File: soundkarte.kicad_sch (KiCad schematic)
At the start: 311 parts, among them J1 JTAG, J2 DB9, J3 Conn_01x05_Pin, J4 Conn_01x06_Pin, J5 Conn_01x08_Pin, J6 LSP R, J7 Sub, J8 LSP L, Q1 Q_NPN_BEC, Q2 BC807, Q3 BC807, U1 DSP56364, U12 LM78M05_TO252, U13 Opamp_Dual, U14 74HC74, U15 TS274CD, U2 28F640, U3 74LS393, U4 74HC14, U8 LD1086D2M33TR, U9 LD1086D2M33TR, X1 SG-8002JC

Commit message: loeschen
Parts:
- removed C1, C2, C3, C4, C47, C48, C49, C5, C50, C51, C6, C7, C8: 220 35G, Capacitor_SMD:CP_Elec_10x10.5, symbol Device:C_Polarized
- removed C10, C11, C12, C13, C14, C15, C16, C17, C18, C27, C28, C29, C30, C31, C32, C33, C34, C35, C36, C37, C38, C39, C40, C41, C42, C43, C44, C45, C46, C55, C56, C57, C61, C62, C63, C64, C65, C66, C67, C68, C69, C70, C73, C74, C9: C, Capacitor_SMD:C_0805_2012Metric, symbol Device:C
- removed C19, C20, C21, C22, C23, C24, C25, C26, C52, C53, C54: 22 35G, Capacitor_SMD:CP_Elec_6.3x3, symbol Device:C_Polarized
- removed C58, C59, C60, C71, C72, C75, C76, C77, C78, C79: C, Capacitor_SMD:C_1206_3216Metric, symbol Device:C
- removed D1, D2, D3, D4: LED, LED_SMD:LED_PLCC-2_3.4x3.0mm_AK, symbol Device:LED
- removed D5: D, Diode_SMD:D_1812_4532Metric, symbol Device:D
- removed FID2, FID3: Fiducial, Fiducial:Fiducial_0.75mm_Mask2.25mm, symbol Mechanical:Fiducial
- removed H5, H6: MountingHole, MountingHole:MountingHole_4mm, symbol Mechanical:MountingHole
- removed H7: MountingHole_Pad, MountingHole:MountingHole_4mm_Pad, symbol Mechanical:MountingHole_Pad
- removed J1: JTAG, Soundkarte:PinHeader_2x7_P1.27mm_Vertical_SMD_Pin1Left, symbol Connector_Generic:Conn_02x07_Odd_Even
- removed J2: DB9, Connector_Dsub:DSUB-9_Female_Vertical_P2.77x2.84mm, symbol Connector:Conn_01x09_Socket
- removed J3: Conn_01x05_Pin, Connector_PinHeader_2.54mm:PinHeader_1x05_P2.54mm_Vertical, symbol Connector:Conn_01x05_Pin
- removed J4: Conn_01x06_Pin, Connector_PinHeader_2.54mm:PinHeader_1x06_P2.54mm_Vertical, symbol Connector:Conn_01x06_Pin
- removed J5: Conn_01x08_Pin, Connector_PinHeader_2.54mm:PinHeader_1x08_P2.54mm_Vertical, symbol Connector:Conn_01x08_Pin
- removed J6: LSP R, Connector_PinHeader_2.54mm:PinHeader_1x02_P2.54mm_Vertical, symbol Connector:Conn_01x02_Pin
- removed J7: Sub, Connector_PinHeader_2.54mm:PinHeader_1x02_P2.54mm_Vertical, symbol Connector:Conn_01x02_Pin
- removed J8: LSP L, Connector_PinHeader_2.54mm:PinHeader_1x02_P2.54mm_Vertical, symbol Connector:Conn_01x02_Pin
- removed JP4: Mcdac, Jumper:SolderJumper-2_P1.3mm_Open_Pad1.0x1.5mm, symbol Jumper:Jumper_2_Open
- removed L1: L_Coupled, Inductor_THT:Choke_Schaffner_RN212-04-12.5x18.0mm, symbol Device:L_Coupled
- removed Q1: Q_NPN_BEC, Package_TO_SOT_SMD:SOT-23-3, symbol Device:Q_NPN_BEC
- removed Q2, Q3: BC807, Package_TO_SOT_SMD:SOT-23-3, symbol Device:Q_PNP_BEC
- removed R1, R10, R11, R12, R13, R14, R15, R16, R17, R18, R19, R2, R20, R21, R22, R23, R24, R25, R26, R27, R28, R29, R3, R30, R31, R34, R35, R36, R37, R38, R4, R44, R45, R46, R49, R5, R51, R52, R53, R54, R55, R56, R57, R58, R6, R7, R8, R9: R, Resistor_SMD:R_0805_2012Metric, symbol Device:R
- removed R32: 0, Resistor_SMD:R_0805_2012Metric, symbol Device:R
- removed R33, R39, R40, R41, R42, R43, R50: 10k, Resistor_SMD:R_0805_2012Metric, symbol Device:R
- removed R47: log, Potentiometer_THT:Potentiometer_ACP_CA6-H2,5_Horizontal, symbol Device:R_Potentiometer
- removed R48: lin, Potentiometer_THT:Potentiometer_ACP_CA6-H2,5_Horizontal, symbol Device:R_Potentiometer
- removed R59, R60, R61, R62, R63, R64: R, Resistor_SMD:R_0603_1608Metric, symbol Device:R
- removed TP10, TP100, TP101, TP102, TP103, TP104, TP105, TP106, TP107, TP108, TP110, TP111, TP112, TP113, TP114, TP115, TP116, TP117, TP118, TP119, TP120, TP121, TP122, TP21, TP50, TP51, TP53, TP54, TP55, TP56, TP57, TP59, TP60, TP61, TP62, TP64, TP65, TP67, TP68, TP70, TP72, TP74, TP75, TP76, TP77, TP78, TP79, TP8, TP80, TP81, TP82, TP83, TP84, TP85, TP86, TP9, TP91, TP93, TP94, TP95, TP96, TP97, TP98, TP99: TestPoint, TestPoint:TestPoint_Pad_D1.0mm, symbol Connector:TestPoint
- removed U1: DSP56364, Package_QFP:LQFP-100_14x14mm_P0.5mm, symbol Soundkarte:DSP56364
- removed U10, U11: ~, Package_SO:SSOP-28_5.3x10.2mm_P0.65mm, symbol Soundkarte:PCM1716
- removed U12: LM78M05_TO252, Package_TO_SOT_SMD:TO-252-2, symbol Regulator_Linear:LM78M05_TO252
- removed U13: Opamp_Dual, Package_SO:SO-8_3.9x4.9mm_P1.27mm, symbol Device:Opamp_Dual
- removed U14: 74HC74, Package_SO:TSSOP-14_4.4x5mm_P0.65mm, symbol 74xx:74HC74
- removed U15: TS274CD, Package_SO:SO-14_3.9x8.65mm_P1.27mm, symbol Amplifier_Operational:TLC274
- removed U2: 28F640, Package_SO:TSOP-I-56_18.4x14mm_P0.5mm, symbol Soundkarte:JS28F640
- removed U3: 74LS393, Package_SO:SO-14_3.9x8.65mm_P1.27mm, symbol 74xx:74LS393
- removed U4: 74HC14, Package_SO:TSSOP-14_4.4x5mm_P0.65mm, symbol 74xx:74HC14
- removed U5, U6, U7: ~, Package_SO:Infineon_PG-DSO-20-87, symbol Soundkarte:TDA7391PD
- removed U8, U9: LD1086D2M33TR, Package_TO_SOT_SMD:TO-263-3_TabPin2, symbol Regulator_Linear:LD1086D2M33TR
- removed X1: SG-8002JC, Oscillator:Oscillator_SMD_SeikoEpson_SG8002JC-4Pin_10.5x5.0mm, symbol Oscillator:SG-8002JC
- added J1: Data, Connector_FFC-FPC:TE_84952-8_1x08-1MP_P1.0mm_Horizontal, symbol Connector_Generic_MountingPin:Conn_01x08_MountingPin
- added J10: Address, Connector_FFC-FPC:TE_2-84952-8_1x28-1MP_P1.0mm_Horizontal, symbol Connector_Generic_MountingPin:Conn_01x28_MountingPin
- added J2: Control, Connector_FFC-FPC:TE_84952-8_1x08-1MP_P1.0mm_Horizontal, symbol Connector_Generic_MountingPin:Conn_01x08_MountingPin
- added J4: Power, Connector_FFC-FPC:TE_84952-8_1x08-1MP_P1.0mm_Horizontal, symbol Connector_Generic_MountingPin:Conn_01x08_MountingPin
- added J5: 1-28, Connector_FFC-FPC:TE_2-84952-8_1x28-1MP_P1.0mm_Horizontal, symbol Connector_Generic_MountingPin:Conn_01x28_MountingPin
- added J6: JTAG, Connector_FFC-FPC:TE_84952-8_1x08-1MP_P1.0mm_Horizontal, symbol Connector_Generic_MountingPin:Conn_01x08_MountingPin
- added J7: 29-56, Connector_FFC-FPC:TE_2-84952-8_1x28-1MP_P1.0mm_Horizontal, symbol Connector_Generic_MountingPin:Conn_01x28_MountingPin
- added J8: Main Power, Connector_Wire:SolderWire-0.25sqmm_1x02_P4.5mm_D0.65mm_OD2mm_Relief, symbol Connector_Generic:Conn_01x02
- added J9: Aux Power, Connector_Wire:SolderWire-0.25sqmm_1x02_P4.5mm_D0.65mm_OD2mm_Relief, symbol Connector_Generic:Conn_01x02
- TP1, TP109, TP11, TP12, TP13, TP14, TP15, TP16, TP17, TP18, TP19, TP2, TP20, TP22, TP23, TP24, TP25, TP26, TP27, TP28, TP29, TP3, TP30, TP31, TP32, TP33, TP34, TP35, TP36, TP37, TP38, TP39, TP4, TP40, TP41, TP42, TP43, TP44, TP45, TP47, TP48, TP49, TP5, TP52, TP58, TP6, TP63, TP66, TP69, TP7, TP71, TP73, TP87, TP88, TP89, TP90, TP92: footprint TestPoint:TestPoint_Pad_D1.0mm -> TestPoint:TestPoint_THTPad_D2.0mm_Drill1.0mm
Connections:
- net +12V: now also J8.1 (Pin_1)
- net +3.3V: now also TP58.1, J4.4 (Pin_4), J4.5 (Pin_5), J4.7 (Pin_7), J5.9 (Pin_9), J6.1 (Pin_1)
- net +5V: now also J9.1 (Pin_1)
- net A0: now also J10.3 (Pin_3), J7.4 (Pin_4)
- net A1: now also J10.4 (Pin_4), J5.28 (Pin_28)
- net A10: now also J10.13 (Pin_13), J5.18 (Pin_18)
- net A11: now also J10.14 (Pin_14), J5.17 (Pin_17)
- net A12: now also J10.15 (Pin_15), J5.13 (Pin_13)
- net A13: now also J10.16 (Pin_16), J5.12 (Pin_12)
- net A14: now also J10.17 (Pin_17), J5.11 (Pin_11)
- net A15: now also J10.18 (Pin_18), J5.10 (Pin_10)
- net A16: now also J10.19 (Pin_19), J5.8 (Pin_8)
- net A17: now also J10.20 (Pin_20), J5.7 (Pin_7)
- net A18: now also J10.21 (Pin_21), J5.6 (Pin_6)
- net A19: now also J10.22 (Pin_22), J5.5 (Pin_5)
- net A2: now also J10.5 (Pin_5), J5.27 (Pin_27)
- net A24: now also J10.27 (Pin_27), J7.28 (Pin_28)
- net A3: now also J10.6 (Pin_6), J5.26 (Pin_26)
- net A4: now also J10.7 (Pin_7), J5.25 (Pin_25)
- net A5: now also J10.8 (Pin_8), J5.24 (Pin_24)
- net A6: now also J10.9 (Pin_9), J5.23 (Pin_23)
- net A7: now also J10.10 (Pin_10), J5.22 (Pin_22)
- net A8: now also J10.11 (Pin_11), J5.20 (Pin_20)
- net A9: now also J10.12 (Pin_12), J5.19 (Pin_19)
- net D0: now also J1.1 (Pin_1), J7.5 (Pin_5)
- net D1: now also J1.2 (Pin_2), J7.7 (Pin_7)
- net D2: now also J1.3 (Pin_3), J7.10 (Pin_10)
- net D3: now also J1.4 (Pin_4), J7.12 (Pin_12)
- net D4: now also J1.5 (Pin_5), J7.16 (Pin_16)
- net D5: now also J1.6 (Pin_6), J7.18 (Pin_18)
- net D6: now also J1.7 (Pin_7), J7.21 (Pin_21)
- net D7: now also J1.8 (Pin_8), J7.23 (Pin_23)
- net GND: now also J1.MP (MountPin), J10.1 (Pin_1), J10.2 (Pin_2), J10.28 (Pin_28), J10.MP (MountPin), J2.3 (Pin_3), J2.MP (MountPin), J4.1 (Pin_1), J4.2 (Pin_2), J4.3 (Pin_3), J4.MP (MountPin), J5.2 (Pin_2), J5.21 (Pin_21), J5.MP (MountPin), J6.3 (Pin_3), J6.7 (Pin_7), J6.MP (MountPin), J7.14 (Pin_14), J7.20 (Pin_20), J7.MP (MountPin), J8.2 (Pin_2), J9.2 (Pin_2)
- net GPIO0: now also J10.23 (Pin_23), J5.4 (Pin_4)
- net GPIO1: now also J10.24 (Pin_24), J5.3 (Pin_3)
- net GPIO2: now also J10.25 (Pin_25), J5.1 (Pin_1)
- net GPIO3: now also J10.26 (Pin_26), J7.2 (Pin_2)
- net RESET: now also J2.7 (Pin_7), J5.16 (Pin_16)
- net TCK: now also J6.4 (Pin_4)
- net TDI: now also J6.2 (Pin_2)
- net TDO: now also J6.6 (Pin_6)
- net TMS: now also J6.8 (Pin_8)
- net MODD: now reaches JP3.1 (A), TP18.1
- net at TP22.1: now also J2.6 (Pin_6), J7.26 (Pin_26)
- net at TP23.1: now also J2.5 (Pin_5), J7.27 (Pin_27)
- net at TP49.1: now also J4.6 (Pin_6), J5.15 (Pin_15)
- net at TP66.1: now also J2.8 (Pin_8), J7.25 (Pin_25)
- net MODA: now reaches JP1.1 (A), TP20.1
- net MODB: now reaches JP2.1 (A), TP19.1
- net at TP47.1: now also J2.2 (Pin_2), J5.14 (Pin_14)
- new net: J2.1 (Pin_1), J2.4 (Pin_4), J7.1 (Pin_1), J7.3 (Pin_3)
- new net: J4.8 (Pin_8), J7.15 (Pin_15), J7.9 (Pin_9)
- no-connect marks 18 -> 0
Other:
- moved on the sheet: TP1, TP11, TP12, TP13, TP14, TP15, TP2, TP3, TP4, TP42, TP43, TP44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

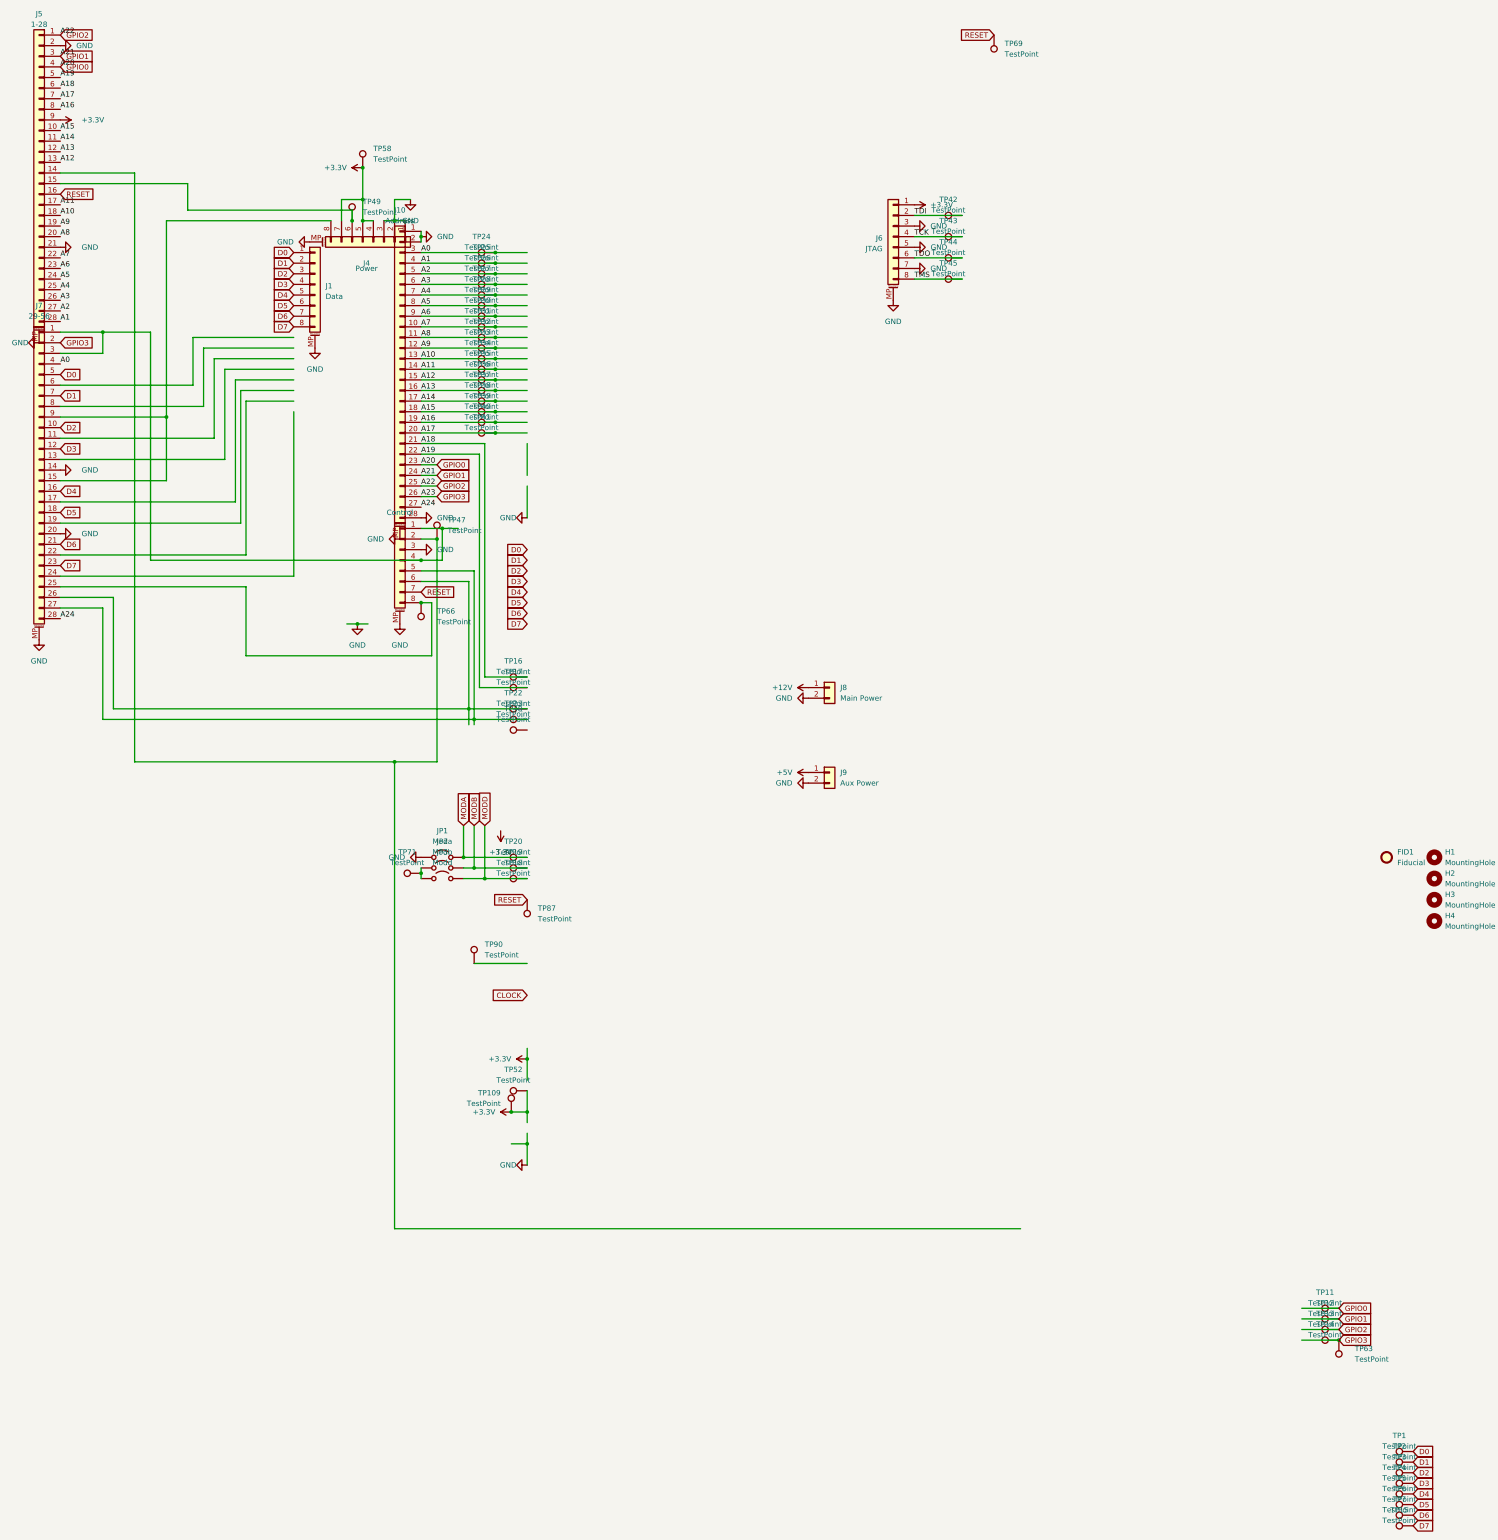
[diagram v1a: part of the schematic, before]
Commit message: teensy
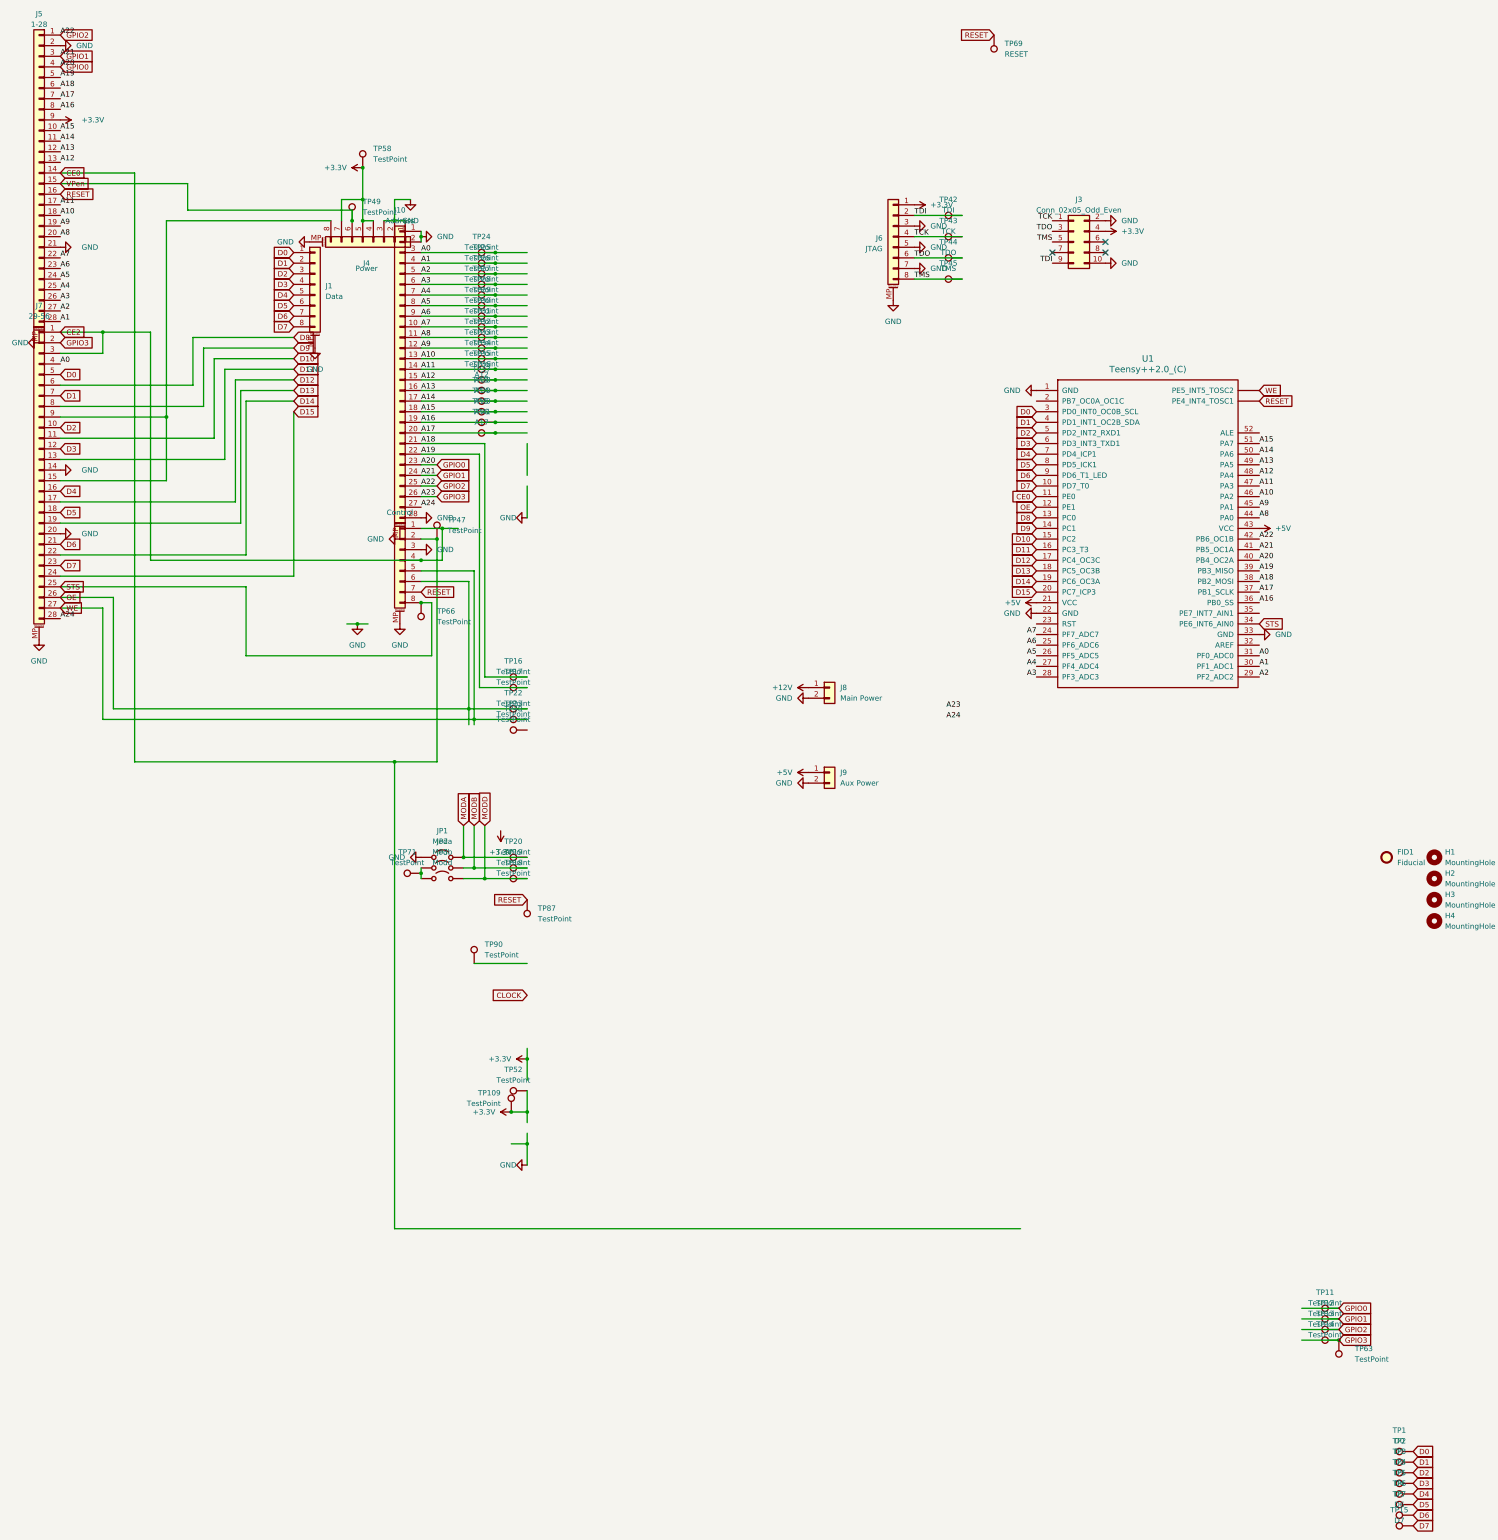
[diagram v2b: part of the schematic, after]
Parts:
- added J3: Conn_02x05_Odd_Even, Connector_PinHeader_2.54mm:PinHeader_2x05_P2.54mm_Vertical, symbol Connector_Generic:Conn_02x05_Odd_Even
- added U1: Teensy++2.0_(C), Soundkarte:Teensy2.0++, symbol teensy:Teensy++2.0_(C)
- TP1: value TestPoint -> D0
- TP15: value TestPoint -> D7
- TP2: value TestPoint -> D1
- TP3: value TestPoint -> D2
- TP36: value TestPoint -> A12
- TP37: value TestPoint -> A13
- TP38: value TestPoint -> A14
- TP39: value TestPoint -> A15
- TP4: value TestPoint -> D3
- TP40: value TestPoint -> A16
- TP41: value TestPoint -> A17
- TP42: value TestPoint -> TDI
- TP43: value TestPoint -> TCK
- TP44: value TestPoint -> TDO
- TP45: value TestPoint -> TMS
- TP5: value TestPoint -> D4
- TP6: value TestPoint -> D5
- TP69: value TestPoint -> RESET
- TP7: value TestPoint -> D6
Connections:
- net +3.3V: now also J3.4 (Pin_4)
- net +5V: now also U1.21 (VCC), U1.43 (VCC)
- net A0: now also U1.31 (PF0_ADC0)
- net A1: now also U1.30 (PF1_ADC1)
- net A10: now also U1.46 (PA2)
- net A11: now also U1.47 (PA3)
- net A12: now also U1.48 (PA4)
- net A13: now also U1.49 (PA5)
- net A14: now also U1.50 (PA6)
- net A15: now also U1.51 (PA7)
- net A16: now also U1.36 (PB0_SS)
- net A17: now also U1.37 (PB1_SCLK)
- net A18: now also U1.38 (PB2_MOSI)
- net A19: now also U1.39 (PB3_MISO)
- net A2: now also U1.29 (PF2_ADC2)
- net A3: now also U1.28 (PF3_ADC3)
- net A4: now also U1.27 (PF4_ADC4)
- net A5: now also U1.26 (PF5_ADC5)
- net A6: now also U1.25 (PF6_ADC6)
- net A7: now also U1.24 (PF7_ADC7)
- net A8: now also U1.44 (PA0)
- net A9: now also U1.45 (PA1)
- net D0: now also U1.3 (PD0_INT0_OC0B_SCL)
- net D1: now also U1.4 (PD1_INT1_OC2B_SDA)
- net D2: now also U1.5 (PD2_INT2_RXD1)
- net D3: now also U1.6 (PD3_INT3_TXD1)
- net D4: now also U1.7 (PD4_ICP1)
- net D5: now also U1.8 (PD5_ICK1)
- net D6: now also U1.9 (PD6_T1_LED)
- net D7: now also U1.10 (PD7_T0)
- net GND: now also J6.5 (Pin_5), J3.10 (Pin_10), J3.2 (Pin_2), U1.1 (GND), U1.22 (GND), U1.33 (GND)
- net GPIO0: now also U1.40 (PB4_OC2A)
- net GPIO1: now also U1.41 (PB5_OC1A)
- net GPIO2: now also U1.42 (PB6_OC1B)
- net RESET: now also U1.~ (PE4_INT4_TOSC1)
- net TCK: now also J3.1 (Pin_1)
- net TDI: now also J3.9 (Pin_9)
- net TDO: now also J3.3 (Pin_3)
- net TMS: now also J3.5 (Pin_5)
- net CE0: now reaches J2.2 (Pin_2), J5.14 (Pin_14), TP47.1
- net CE0: now also U1.11 (PE0)
- net VPen: now reaches J4.6 (Pin_6), J5.15 (Pin_15), TP49.1
- net CE2: now reaches J2.1 (Pin_1), J2.4 (Pin_4), J7.1 (Pin_1), J7.3 (Pin_3)
- net WE: now reaches J2.5 (Pin_5), J7.27 (Pin_27), TP23.1
- net WE: now also U1.~ (PE4_INT4_TOSC1)
- net OE: now reaches J2.6 (Pin_6), J7.26 (Pin_26), TP22.1
- net OE: now also U1.12 (PE1)
- net STS: now reaches J2.8 (Pin_8), J7.25 (Pin_25), TP66.1
- net STS: now also U1.34 (PE6_INT6_AIN0)
- net D10: now reaches J7.11 (Pin_11)
- net D10: now also U1.15 (PC2)
- net D11: now reaches J7.13 (Pin_13)
- net D11: now also U1.16 (PC3_T3)
- net D12: now reaches J7.17 (Pin_17)
- net D12: now also U1.17 (PC4_OC3C)
- net D13: now reaches J7.19 (Pin_19)
- net D13: now also U1.18 (PC5_OC3B)
- net D14: now reaches J7.22 (Pin_22)
- net D14: now also U1.19 (PC6_OC3A)
- net D15: now reaches J7.24 (Pin_24)
- net D15: now also U1.20 (PC7_ICP3)
- net D8: now reaches J7.6 (Pin_6)
- net D8: now also U1.13 (PC0)
- net D9: now reaches J7.8 (Pin_8)
- net D9: now also U1.14 (PC1)
- no-connect marks 0 -> 3
